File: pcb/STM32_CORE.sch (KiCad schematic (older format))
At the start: 34 parts, among them J11 Conn_01x04, J12 Conn_01x04, J6 Conn_01x14, J7 Conn_01x12, J8 Conn_01x15, SW1 SW_Push, U3 STM32F103C8T6, U4 AMS1117-3.3, Y1 O8M, Y2 O_EPSON_32.768K

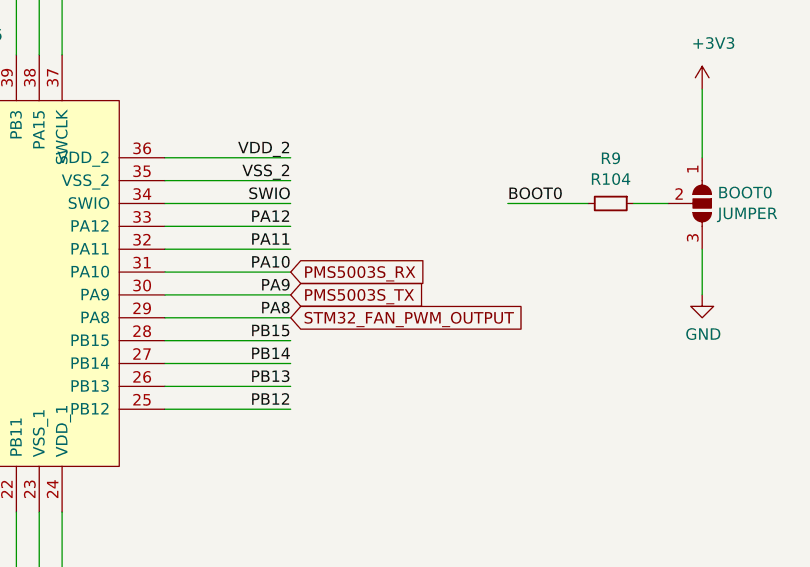
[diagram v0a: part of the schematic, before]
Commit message: update,
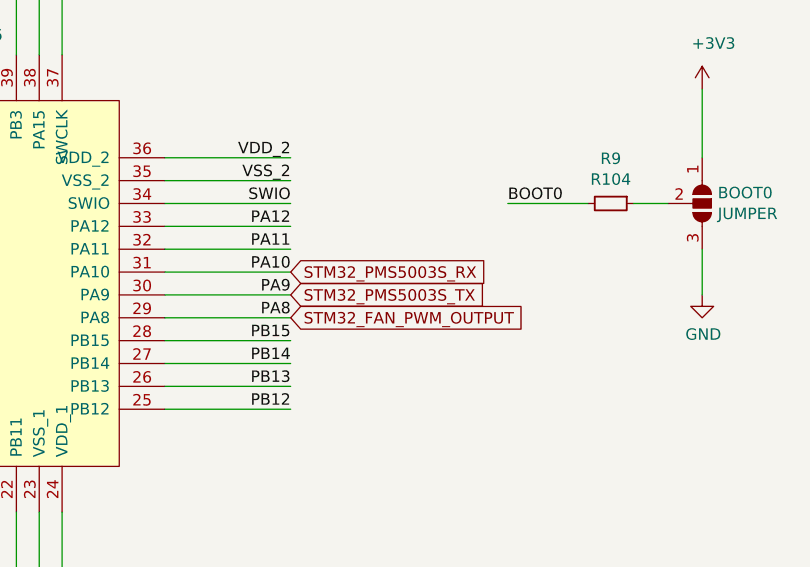
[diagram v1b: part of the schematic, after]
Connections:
- net labels added: STM32_PMS5003S_RX, STM32_PMS5003S_TX
- net labels removed: PMS5003S_RX, PMS5003S_TX
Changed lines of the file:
@@
 $Descr A3 16535 11693
 encoding utf-8
-Sheet 5 7
+Sheet 5 8
 Title ""
 Date ""
@@
 	11050 5350 11050 5550
 Text GLabel 10000 3150 2    50   Input ~ 0
-PMS5003S_RX
+STM32_PMS5003S_RX
 Text GLabel 10000 3250 2    50   Input ~ 0
-PMS5003S_TX
+STM32_PMS5003S_TX
 Text Label 6550 1400 2    50   ~ 0
 VBAT
@@
 	6100 1500 6100 1400
 $Comp
-L power:GND #PWR?
+L power:GND #PWR0116
 U 1 1 5BDB5D1B
 P 6100 2300
-F 0 "#PWR?" H 6100 2050 50  0001 C CNN
+F 0 "#PWR0116" H 6100 2050 50  0001 C CNN
 F 1 "GND" H 6105 2127 50  0000 C CNN
 F 2 "" H 6100 2300 50  0001 C CNN

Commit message: update,
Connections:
- net labels added: B2B_UART_RX, B2B_UART_TX, STM32_PMS7003S_RESET, STM32_PMS7003S_RXD, STM32_PMS7003S_SET, STM32_PMS7003S_TXD
- net labels removed: STM32_PMS5003S_RX, STM32_PMS5003S_TX
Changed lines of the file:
@@
 	11050 5350 11050 5550
 Text GLabel 10000 3150 2    50   Input ~ 0
-STM32_PMS5003S_RX
+STM32_PMS7003S_RXD
 Text GLabel 10000 3250 2    50   Input ~ 0
-STM32_PMS5003S_TX
+STM32_PMS7003S_TXD
 Text Label 6550 1400 2    50   ~ 0
 VBAT
@@
 Wire Wire Line
 	6100 2100 6100 2000
+Text GLabel 10000 2950 2    50   Input ~ 0
+STM32_PMS7003S_RESET
+Text GLabel 10000 3050 2    50   Input ~ 0
+STM32_PMS7003S_SET
+Text GLabel 8700 4750 3    50   Input ~ 0
+B2B_UART_TX
+Text GLabel 8800 4750 3    50   Input ~ 0
+B2B_UART_RX
 $EndSCHEMATC
